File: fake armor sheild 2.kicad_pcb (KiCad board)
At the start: 2 copper layers, 134 x 124.5 mm, 47 parts, among them SW1 SW_Nidec_CAS-120A1, SW2 SW_Nidec_CAS-120A1

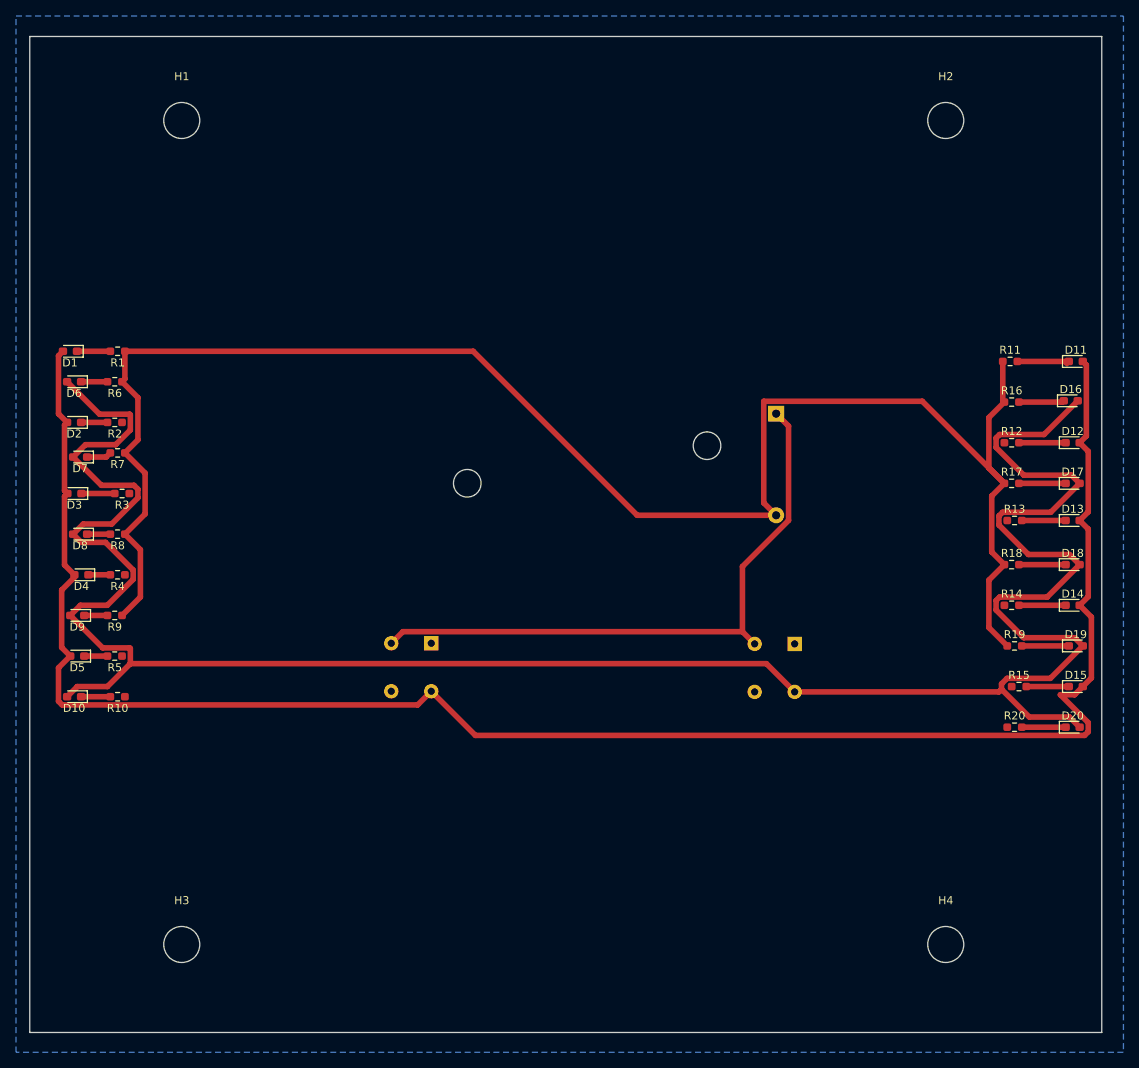
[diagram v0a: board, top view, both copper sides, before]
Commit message: Add files via upload
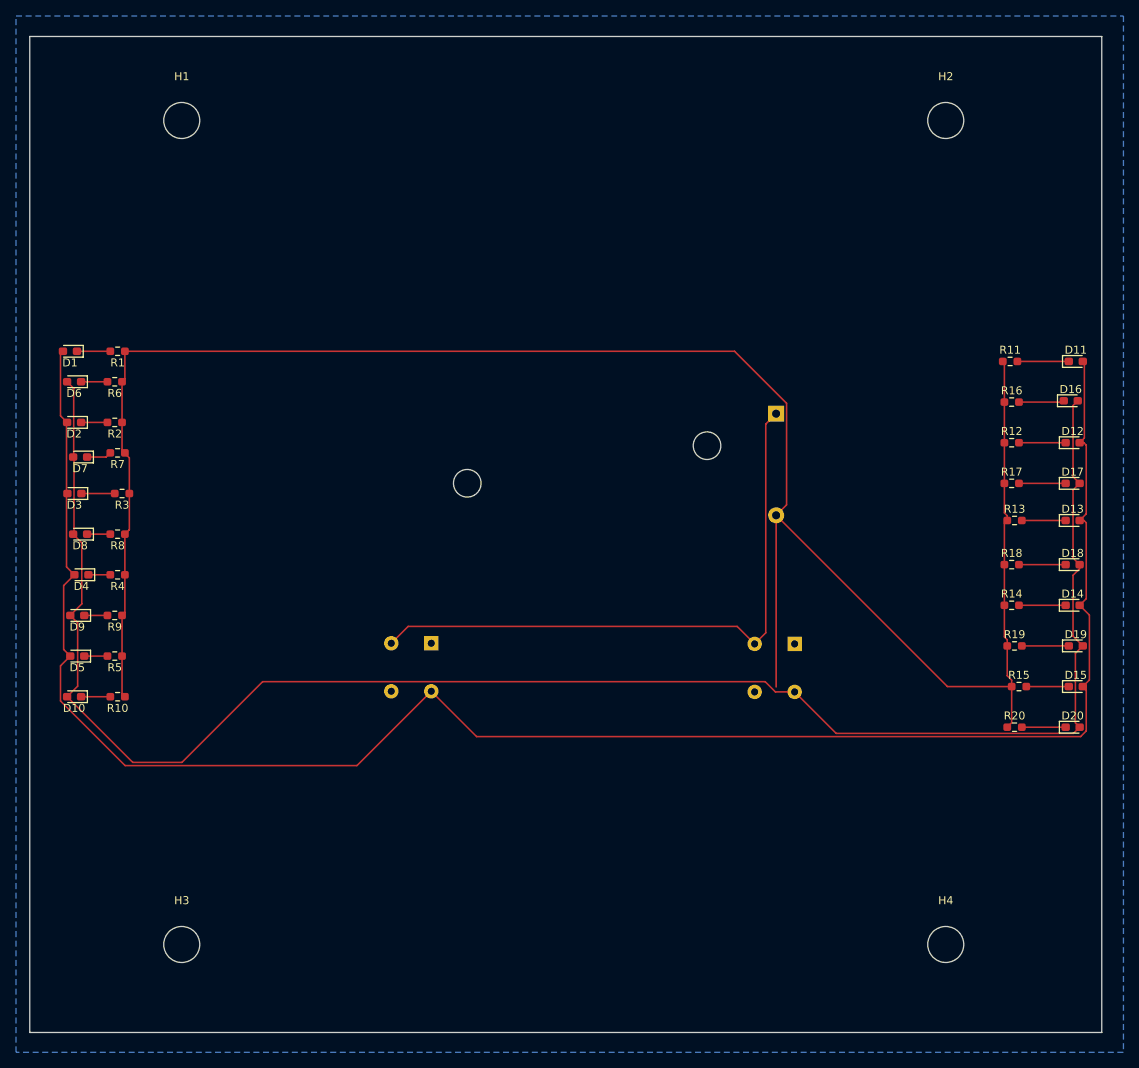
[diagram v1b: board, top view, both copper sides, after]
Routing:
- net /3V blue: track 293.8 -> 222.6 mm
- net GND: track 217.9 -> 250.6 mm
- net /3V Red: track 232.5 -> 233.7 mm
